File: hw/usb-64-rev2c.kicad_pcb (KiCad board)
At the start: 4 copper layers, 62.2 x 43.2 mm, 75 parts, among them J1 USB_C_Receptacle_PowerOnly_6P, J100 Conn_01x03_Pin, J2 USB_C_Receptacle_USB2.0_14P, J3 USB_C_Receptacle_USB2.0_14P, J300 DE9_Receptacle, J301 DE9_Receptacle, SW1 SW_Push, SW2 SW_Push, U100 NCP1117-3.3, U200 RP2040, U201 W25Q128JVSIQ, U300 74AHCT1G125, U301 74AHCT1G125, U302 74AHCT1G125, U303 74AHCT1G125, U304 74AHCT1G125, U305 74AHCT1G125, U306 74AHCT1G125, U307 74AHCT1G125, U308 74AHCT1G125, U309 74AHCT1G125, X100 ASE-12MHz

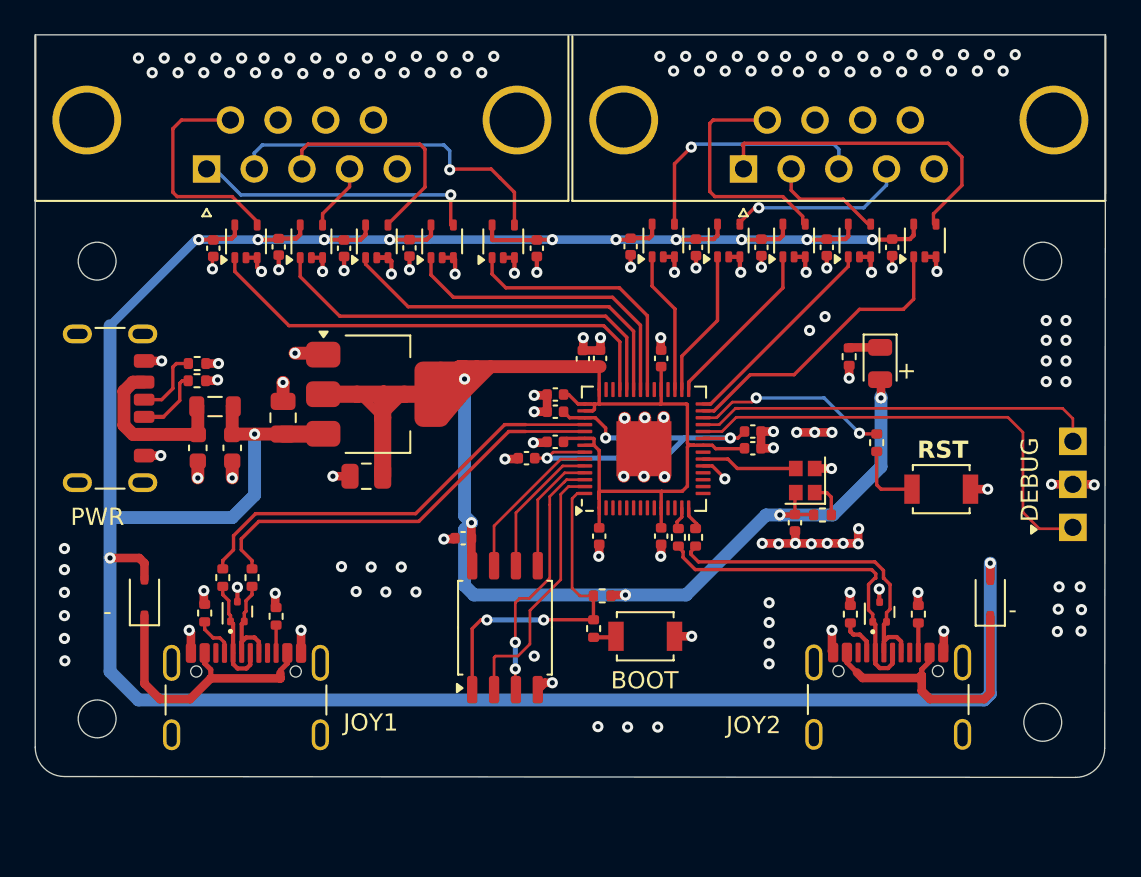
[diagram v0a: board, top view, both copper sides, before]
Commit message: 1p version
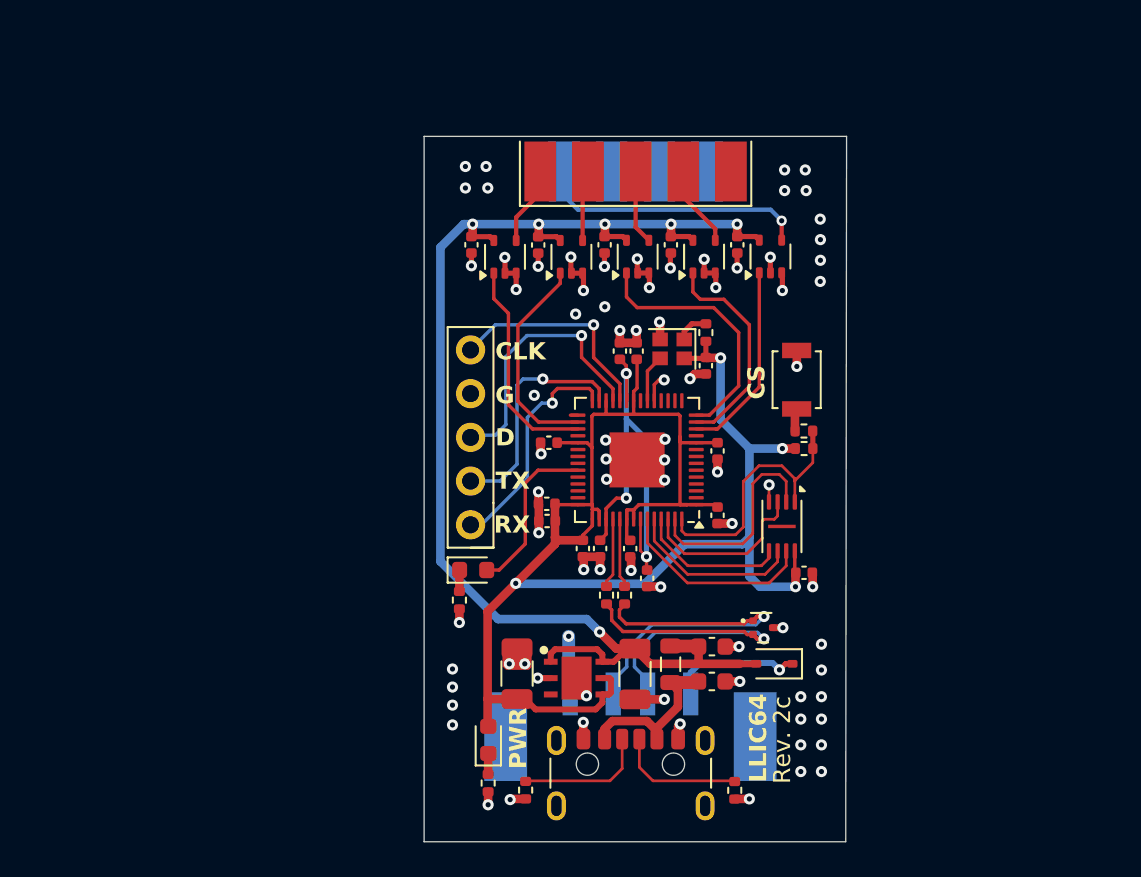
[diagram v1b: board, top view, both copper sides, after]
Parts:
- removed ?: , clipboard:7c1455c2-a98c-4e40-9696-5f6f5e7dbb40
- removed C100, C101: 10u, Capacitor_SMD:C_0805_2012Metric
- removed C305, C306, C307, C308, C309: 100n, Capacitor_SMD:C_0402_1005Metric
- removed D3: ESD7L5.0DT5G, Package_TO_SOT_SMD:SOT-723
- removed D4, D5: 40V 600mV@1A 1A, Diode_SMD:D_SOD-323
- removed H1, H2, H3, H4: MountingHole, MountingHole:MountingHole_2.2mm_M2
- removed J3: USB_C_Receptacle_USB2.0_14P, Connector_USB:USB_C_Receptacle_GCT_USB4105-xx-A_16P_TopMnt_Horizontal
- removed J301: DE9_Receptacle, Connector_Dsub:DSUB-9_Female_Horizontal_P2.77x2.84mm_EdgePinOffset4.94mm_Housed_MountingHolesOffset4.94mm
- removed R1, R208: 1k, Resistor_SMD:R_0402_1005Metric
- removed R2, R3, R4, R5: 5K1, Resistor_SMD:R_0402_1005Metric
- removed R205, R206: 27R, Resistor_SMD:R_0402_1005Metric
- removed SW2: SW_Push, Button_Switch_SMD:SW_SPST_B3U-1000P
- removed U100: NCP1117-3.3, Package_TO_SOT_SMD:SOT-223-3_TabPin2
- removed U305, U306, U307, U308, U309: 74AHCT1G125, Package_TO_SOT_SMD:SOT-353_SC-70-5
- added C3: 4.7u, Capacitor_SMD:C_1206_3216Metric, F.Cu at (150.9, 86.1)
- added C4: 4.7u, Capacitor_SMD:C_1206_3216Metric, F.Cu at (144.1, 86.1)
- added D6: RED, LED_SMD:LED_0603_1608Metric, F.Cu at (142.4, 90.0)
- added D7: RED, LED_SMD:LED_0603_1608Metric, F.Cu at (141.5, 80.1)
- added IC1: NCP708MU330TAG, Package_SON:SON95P300X300X55-7N, F.Cu at (147.5, 86.4)
- added R6: 330, Resistor_SMD:R_0402_1005Metric, F.Cu at (142.4, 92.5)
- added R9: 330, Resistor_SMD:R_0402_1005Metric, F.Cu at (140.7, 81.8)
- D1: value GREEN -> ESD7L5.0DT5G; footprint LED_SMD:LED_0805_2012Metric -> Package_TO_SOT_SMD:SOT-723
- D2: value ESD7L5.0DT5G -> D_Schottky; footprint Package_TO_SOT_SMD:SOT-723 -> Diode_SMD:D_SOD-323
- J100: value Conn_01x03_Pin -> Conn_01x05_Pin; footprint Connector_PinHeader_2.54mm:PinHeader_1x03_P2.54mm_Vertical -> Connector_PinHeader_2.54mm:PinHeader_1x05_P2.54mm_Vertical
- J2: value USB_C_Receptacle_USB2.0_14P -> USB_A; footprint Connector_USB:USB_C_Receptacle_GCT_USB4105-xx-A_16P_TopMnt_Horizontal -> Connector_USB:CONN_UJ2-AH-SMT_CUD; moved to B.Cu
- J300: footprint Connector_Dsub:DSUB-9_Female_Horizontal_P2.77x2.84mm_EdgePinOffset4.94mm_Housed_MountingHolesOffset4.94mm -> Connector_Dsub:DSUB-9_Female_EdgeMount_P2.77mm
- U201: value W25Q128JVSIQ -> W25Q16JVUXIQ; footprint Package_SO:SOIC-8_5.23x5.23mm_P1.27mm -> Package_SON:Winbond_USON-8-1EP_3x2mm_P0.5mm_EP0.2x1.6mm
- moved R7 39.3 mm to (156.7, 92.9), turned to -90 degrees
- moved J1 38.5 mm to (150.7, 93.0), turned to 0 degrees
- moved J100 35.3 mm to (141.3, 77.5), turned to 180 degrees
- moved C1 32.8 mm to (155.4, 86.6), turned to 0 degrees
- moved D2 31.3 mm to (159.0, 85.5), turned to 180 degrees
- moved R8 31.3 mm to (144.6, 92.9), turned to -90 degrees
- moved U304 30.5 mm to (158.8, 61.9)
- moved FB3 30.4 mm to (153.0, 85.6), turned to 90 degrees
- moved C2 30.2 mm to (155.4, 84.5), turned to 0 degrees
- moved C303 26.7 mm to (156.8, 61.2)
- moved J300 24.9 mm to (150.9, 56.9)
- moved U303 22.8 mm to (154.9, 61.9)
- moved R201 22.3 mm to (149.2, 81.6), turned to -90 degrees
- moved R200 21.7 mm to (150.3, 81.6), turned to -90 degrees
- moved C214 19.9 mm to (160.7, 80.3), turned to 180 degrees
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- renumbered C5 to C1, C6 to C2
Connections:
- C1 pad 1: VBUS -> Net-(C1-Pad1)
- D1 pad 1: Net-(D1-K) -> /USB_MCU_D_P
- D1 pad 2: +3.3V -> /USB_MCU_D_N
- D2 pad 1: USB_MCU_D_N -> Net-(D2-K)
- D2 pad 2: USB_MCU_D_P -> VBUS
- FB3 pad 1: VBUS -> Net-(C1-Pad1)
- J1 pad A9: VBUS -> Net-(C1-Pad1)
- J1 pad B9: VBUS -> Net-(C1-Pad1)
- J100 pad 1: /MCU/SWD -> /MCU/UART_RX
- J100 pad 2: GND -> /MCU/UART_TX
- J100 pad 3: /MCU/SWCLK -> /MCU/SWD
- R200 pad 1: USB_MCU_D_P -> /USB_MCU_D_P
- R200 pad 2: USB_MCU_D_P -> /USB_MCU_D_P
- R201 pad 1: USB_MCU_D_N -> /USB_MCU_D_N
- R201 pad 2: USB_MCU_D_N -> /USB_MCU_D_N
- U200 pad 12: unconnected-(U200-GPIO9-Pad12) -> /C64_controls/IO_FIRE
- U200 pad 13: USB_DEV_D_N -> /C64_controls/IO_RIGHT
- U200 pad 14: USB_DEV_D_P -> /C64_controls/IO_LEFT
- U200 pad 26: /MCU/RUN -> +3.3V
- U200 pad 27: IO2_UP -> /MCU/UART_TX
- U200 pad 28: IO2_DOWN -> /MCU/UART_RX
- U200 pad 29: IO2_FIRE -> unconnected-(U200-GPIO18-Pad29)
- U200 pad 30: IO2_RIGHT -> /C64_controls/IO_DOWN
- U200 pad 31: IO2_LEFT -> /C64_controls/IO_UP
- U200 pad 35: IO_DOWN -> unconnected-(U200-GPIO23-Pad35)
- U200 pad 36: IO_UP -> unconnected-(U200-GPIO24-Pad36)
- U200 pad 37: IO_LEFT -> /MCU/GPIO25
- U200 pad 38: IO_RIGHT -> unconnected-(U200-GPIO26_ADC0-Pad38)
- U200 pad 39: IO_FIRE -> unconnected-(U200-GPIO27_ADC1-Pad39)
- U200 pad 46: USB_MCU_D_N -> /USB_MCU_D_N
- U200 pad 47: USB_MCU_D_P -> /USB_MCU_D_P
- U300 pad 1: IO_UP -> /C64_controls/IO_UP
- U301 pad 1: IO_DOWN -> /C64_controls/IO_DOWN
- U302 pad 1: IO_LEFT -> /C64_controls/IO_LEFT
- U303 pad 1: IO_RIGHT -> /C64_controls/IO_RIGHT
- U304 pad 1: IO_FIRE -> /C64_controls/IO_FIRE
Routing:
- net VBUS: track 191.4 -> 76.4 mm, vias 13 -> 6
- net USB_MCU_D_N: track 31.9 -> 0.00 mm
- net USB_MCU_D_P: track 31.2 -> 0.00 mm
- net GND: track 85.3 -> 54.2 mm, vias 170 -> 82
- net IO_FIRE: track 27.6 -> 0.00 mm
- net /USB_MCU_D_P: track 0.00 -> 25.6 mm, vias 0 -> 1
- net /USB_MCU_D_N: track 0.00 -> 25.3 mm, vias 0 -> 1
- net IO_RIGHT: track 24.6 -> 0.00 mm
- net USB_DEV_D_P: track 21.2 -> 0.00 mm
- net USB_DEV_D_N: track 21.2 -> 0.00 mm
- net IO_LEFT: track 21.0 -> 0.00 mm
- net /C64_controls/JOY2_UP: track 19.1 -> 0.00 mm
- net +3.3V: track 121.7 -> 102.6 mm, vias 5 -> 4
- net IO_UP: track 18.1 -> 0.00 mm
- net IO2_UP: track 17.4 -> 0.00 mm
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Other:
- board size 62.2 x 43.2 mm -> 24.5 x 41 mm
- board text added: "CLK"
- board text added: "CS"
- board text added: "D"
- board text added: "G"
- board text added: "LLIC64"
- board text added: "RX"
- board text added: "Rev. 2c"
- board text added: "TX"
- board text added: "github.com/marcopiovanello"
- board text removed: "+"
- board text removed: "-"
- board text removed: "BOOT"
- board text removed: "Control port USB converter"
- board text removed: "DEBUG"
- board text removed: "JOY1"
- board text removed: "JOY2"
- board text removed: "RST"
- board text removed: "USB64"
- board text removed: "github.com/marcopiovanello/usb64"
